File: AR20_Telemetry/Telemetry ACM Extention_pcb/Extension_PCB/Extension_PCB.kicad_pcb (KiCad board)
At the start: 2 copper layers, 55 x 75.5 mm, 9 parts, among them IC1 MCP25625T-E_ML

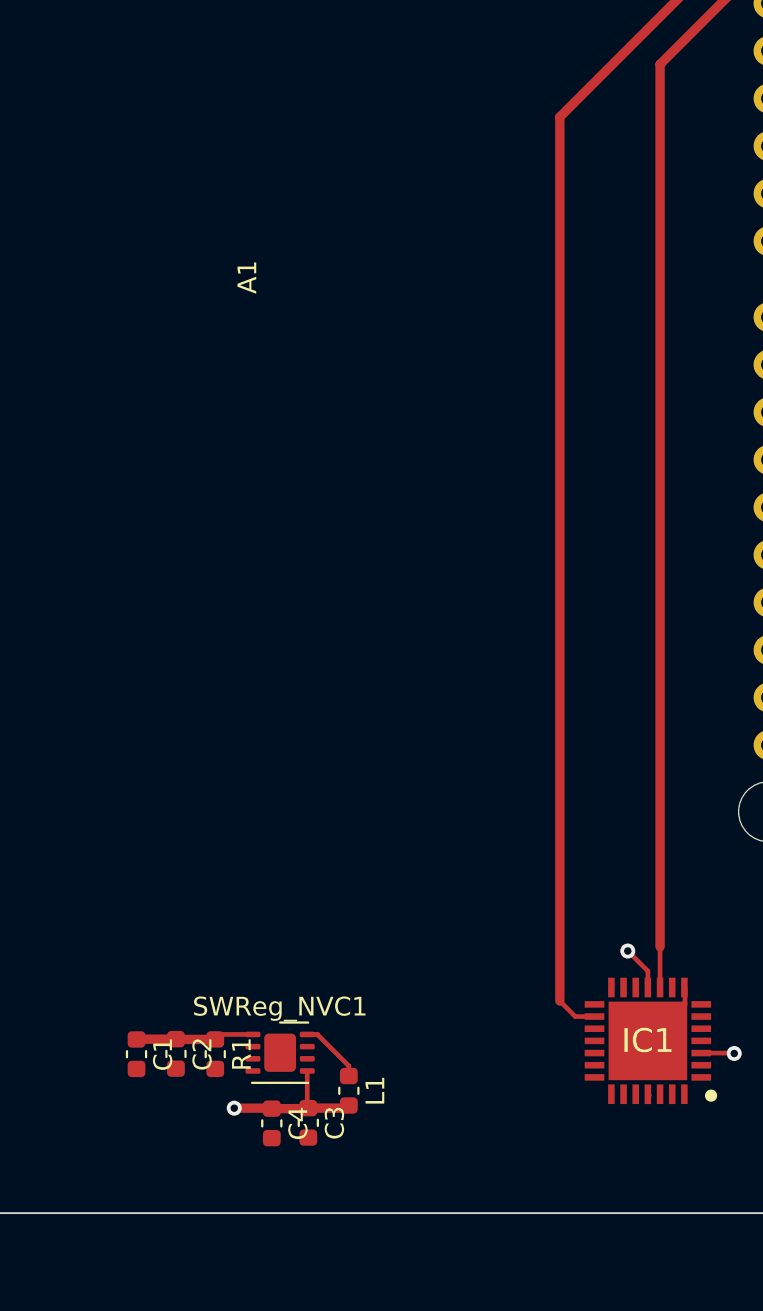
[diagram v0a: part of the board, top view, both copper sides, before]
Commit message: Edited
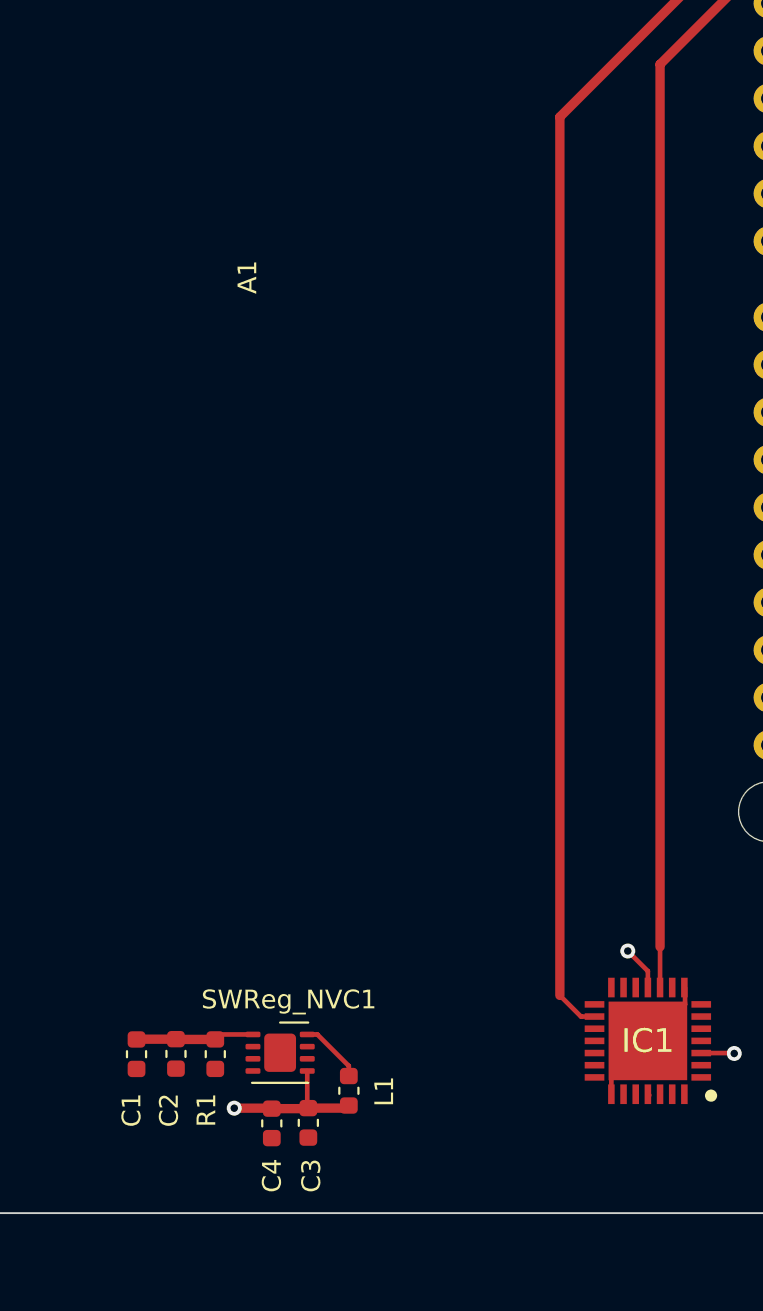
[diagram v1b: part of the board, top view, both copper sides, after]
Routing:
- net Ground: track 3.66 -> 7.32 mm
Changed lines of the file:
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@@
     (thickness 1.6)
     (drawings 4)
-    (tracks 37)
+    (tracks 39)
     (zones 0)
     (modules 9)
@@
     (47 F.CrtYd user)
     (48 B.Fab user)
-    (49 F.Fab user)
+    (49 F.Fab user hide)
   )
   (setup
@@
       (effects (font (size 1.27 1.27) (thickness 0.254)))
     )
-    (fp_text value MCP25625T-E_ML (at 0 0) (layer F.SilkS) hide
+    (fp_text value MCP25625T-E_ML (at 0.57366 -5.19992) (layer F.SilkS) hide
       (effects (font (size 1.27 1.27) (thickness 0.254)))
     )
@@
     (tags "DFN DFN_QFN")
     (attr smd)
-    (fp_text reference SWReg_NVC1 (at 0 -2.45) (layer F.SilkS)
-      (effects (font (size 1 1) (thickness 0.15)))
-    )
-    (fp_text value NCV890430MW50TXG (at 0.6663 7.2878) (layer F.Fab)
-      (effects (font (size 1 1) (thickness 0.15)))
-    )
-    (fp_text user %R (at 0 0) (layer F.Fab)
+    (fp_text reference SWReg_NVC1 (at 0.47152 -2.832) (layer F.SilkS)
+      (effects (font (size 1 1) (thickness 0.15)))
+    )
+    (fp_text value NCV890430MW50TXG (at -0.42848 -6.432) (layer F.Fab)
+      (effects (font (size 1 1) (thickness 0.15)))
+    )
+    (fp_text user %R (at 7.07152 -1.432) (layer F.Fab)
       (effects (font (size 0.75 0.75) (thickness 0.11)))
     )
@@
     (tags resistor)
     (attr smd)
-    (fp_text reference R1 (at 0 -1.43 90) (layer F.SilkS)
-      (effects (font (size 1 1) (thickness 0.15)))
-    )
-    (fp_text value 10k (at 0 1.43 90) (layer F.Fab)
+    (fp_text reference R1 (at 2.99136 0.46474 90) (layer F.SilkS)
+      (effects (font (size 1 1) (thickness 0.15)))
+    )
+    (fp_text value 10k (at -3.00864 -0.03526 90) (layer F.Fab)
       (effects (font (size 1 1) (thickness 0.15)))
     )
@@
     (tags inductor)
     (attr smd)
-    (fp_text reference L1 (at 0 -1.43 90) (layer F.SilkS)
-      (effects (font (size 1 1) (thickness 0.15)))
-    )
-    (fp_text value 2.2u (at 0 1.43 90) (layer F.Fab)
+    (fp_text reference L1 (at 0.03556 -1.9004 90) (layer F.SilkS)
+      (effects (font (size 1 1) (thickness 0.15)))
+    )
+    (fp_text value 2.2u (at 0 -3.4004 90) (layer F.Fab)
       (effects (font (size 1 1) (thickness 0.15)))
     )
@@
     (tags capacitor)
     (attr smd)
-    (fp_text reference C4 (at 0 -1.43 90) (layer F.SilkS)
-      (effects (font (size 1 1) (thickness 0.15)))
-    )
-    (fp_text value 10u (at 0 1.43 90) (layer F.Fab)
-      (effects (font (size 1 1) (thickness 0.15)))
-    )
-    (fp_text user %R (at 0 0 90) (layer F.Fab)
+    (fp_text reference C4 (at 2.79312 -0.0152 90) (layer F.SilkS)
+      (effects (font (size 1 1) (thickness 0.15)))
+    )
+    (fp_text value 10u (at 2.29312 1.9848 90) (layer F.Fab)
+      (effects (font (size 1 1) (thickness 0.15)))
+    )
+    (fp_text user %R (at 0.19312 1.2848 90) (layer F.Fab)
       (effects (font (size 0.4 0.4) (thickness 0.06)))
     )
@@
     (tags capacitor)
     (attr smd)
-    (fp_text reference C3 (at 0 -1.43 90) (layer F.SilkS)
-      (effects (font (size 1 1) (thickness 0.15)))
-    )
-    (fp_text value 0.1u (at 0 1.43 90) (layer F.Fab)
+    (fp_text reference C3 (at 2.82086 -0.16448 90) (layer F.SilkS)
+      (effects (font (size 1 1) (thickness 0.15)))
+    )
+    (fp_text value 0.1u (at 2.82086 -0.06448 90) (layer F.Fab)
       (effects (font (size 0.7 0.7) (thickness 0.1)))
     )
-    (fp_text user %R (at 0 0 90) (layer F.Fab)
+    (fp_text user %R (at 0.02086 -1.16448 90) (layer F.Fab)
       (effects (font (size 0.4 0.4) (thickness 0.06)))
     )
@@
     (tags capacitor)
     (attr smd)
-    (fp_text reference C2 (at 0 -1.43 90) (layer F.SilkS)
-      (effects (font (size 1 1) (thickness 0.15)))
-    )
-    (fp_text value 0.1u (at 0 1.43 90) (layer F.Fab)
+    (fp_text reference C2 (at 3.00386 0.36416 90) (layer F.SilkS)
+      (effects (font (size 1 1) (thickness 0.15)))
+    )
+    (fp_text value 0.1u (at -3.49614 -0.13584 90) (layer F.Fab)
       (effects (font (size 1 1) (thickness 0.15)))
     )
@@
     (tags capacitor)
     (attr smd)
-    (fp_text reference C1 (at 0 -1.43 90) (layer F.SilkS)
-      (effects (font (size 1 1) (thickness 0.15)))
-    )
-    (fp_text value 10u (at 0 1.43 90) (layer F.Fab)
+    (fp_text reference C1 (at 2.98862 0.2585 90) (layer F.SilkS)
+      (effects (font (size 1 1) (thickness 0.15)))
+    )
+    (fp_text value 10u (at -3.01138 0.2585 90) (layer F.Fab)
       (effects (font (size 1 1) (thickness 0.15)))
     )
@@
   (gr_line (start 145 147) (end 200 147) (layer Edge.Cuts) (width 0.1))
   (gr_line (start 145 71.5) (end 145 147) (layer Edge.Cuts) (width 0.1))
+  (segment (start 190.6524 140.70342) (end 190.60922 140.66024) (width 0.25) (layer F.Cu) (net 0))
+  (segment (start 187.73406 137.1854) (end 187.75922 137.16024) (width 0.25) (layer F.Cu) (net 0))
   (segment (start 192.55922 135.86024) (end 190.60922 137.81024) (width 0.25) (layer F.Cu) (net 1))
   (segment (start 192.55922 134.96024) (end 192.55922 135.86024) (width 0.25) (layer F.Cu) (net 1))
+  (segment (start 188.62366 139.75008) (end 190.57366 137.80008) (width 0.25) (layer F.Cu) (net 1))
+  (segment (start 188.62366 140.65008) (end 188.62366 139.75008) (width 0.25) (layer F.Cu) (net 1))
   (segment (start 165.37666 137.72114) (end 165.36416 137.70864) (width 0.5) (layer F.Cu) (net 2))
   (segment (start 167.46474 137.72114) (end 165.37666 137.72114) (width 0.5) (layer F.Cu) (net 2))
   (segment (start 163.27374 137.70864) (end 163.2585 137.72388) (width 0.5) (layer F.Cu) (net 2))
   (segment (start 165.36416 137.70864) (end 163.27374 137.70864) (width 0.5) (layer F.Cu) (net 2))
-  (segment (start 174.5869 139.66424) (end 174.5996 139.67694) (width 0.5) (layer F.Cu) (net 3))
-  (via (at 195.1863 138.47318) (size 0.8) (drill 0.4) (layers F.Cu B.Cu) (net 7))
-  (via (at 168.4782 141.39418) (size 0.8) (drill 0.4) (layers F.Cu B.Cu) (net 7))
-  (segment (start 190.6524 140.70342) (end 190.60922 140.66024) (width 0.25) (layer F.Cu) (net 0))
-  (segment (start 187.73406 137.1854) (end 187.75922 137.16024) (width 0.25) (layer F.Cu) (net 0))
   (segment (start 167.72888 137.457) (end 167.46474 137.72114) (width 0.25) (layer F.Cu) (net 2))
   (segment (start 169.47848 137.457) (end 167.72888 137.457) (width 0.25) (layer F.Cu) (net 2))
+  (segment (start 174.5869 139.66424) (end 174.5996 139.67694) (width 0.5) (layer F.Cu) (net 3))
   (segment (start 174.5996 139.13944) (end 174.5996 139.67694) (width 0.25) (layer F.Cu) (net 3))
   (segment (start 172.91716 137.457) (end 174.5996 139.13944) (width 0.25) (layer F.Cu) (net 3))
@@
   (segment (start 191.22366 132.77634) (end 191.22366 85.63634) (width 0.5) (layer F.Cu) (net 5))
   (segment (start 196.220181 78.099819) (end 197.02018 77.29982) (width 0.5) (layer F.Cu) (net 6))
+  (segment (start 185.87212 135.37212) (end 185.87212 88.44788) (width 0.5) (layer F.Cu) (net 6))
   (segment (start 185.87212 88.44788) (end 196.220181 78.099819) (width 0.5) (layer F.Cu) (net 6))
-  (segment (start 185.87212 135.67354) (end 185.87212 88.44788) (width 0.5) (layer F.Cu) (net 6))
-  (segment (start 186.69866 136.50008) (end 185.87212 135.67354) (width 0.25) (layer F.Cu) (net 6))
-  (segment (start 187.72366 136.50008) (end 186.69866 136.50008) (width 0.25) (layer F.Cu) (net 6))
+  (segment (start 187.00008 136.50008) (end 185.87212 135.37212) (width 0.25) (layer F.Cu) (net 6))
+  (segment (start 187.72366 136.50008) (end 187.00008 136.50008) (width 0.25) (layer F.Cu) (net 6))
+  (via (at 195.1863 138.47318) (size 0.8) (drill 0.4) (layers F.Cu B.Cu) (net 7))
+  (via (at 168.4782 141.39418) (size 0.8) (drill 0.4) (layers F.Cu B.Cu) (net 7))
   (segment (start 170.4596 141.39418) (end 170.4848 141.41938) (width 0.5) (layer F.Cu) (net 7))
   (segment (start 168.4782 141.39418) (end 170.4596 141.39418) (width 0.5) (layer F.Cu) (net 7))

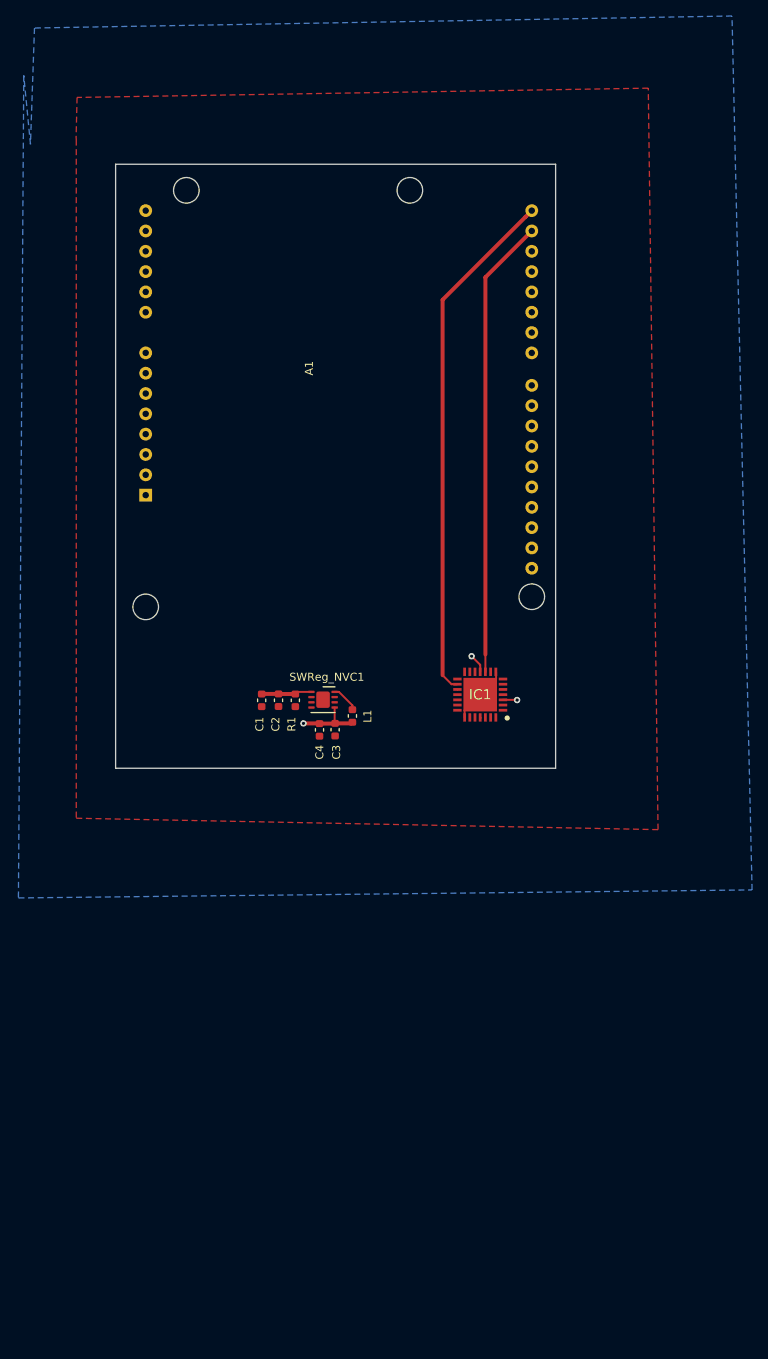
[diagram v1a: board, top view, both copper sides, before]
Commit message: Connector added
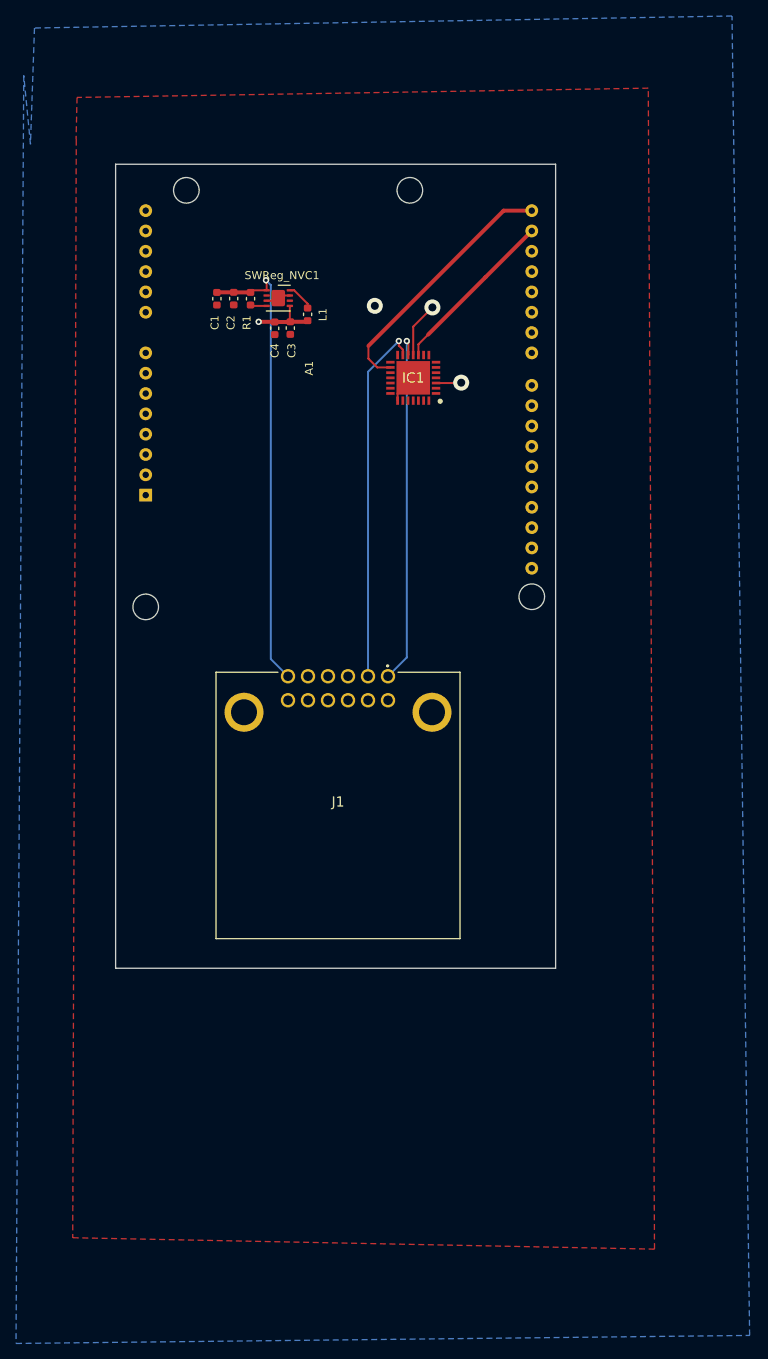
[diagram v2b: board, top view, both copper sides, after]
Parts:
- added J1: MX23A12NF1, MCP25625_Breakoutboard:MX23A12NF1, F.Cu at (172.8, 151.2)
- moved C4 50.5 mm to (164.9, 92.0)
- moved R1 50.5 mm to (161.9, 88.3)
- moved C1 50.5 mm to (157.7, 88.3)
- moved C2 50.5 mm to (159.8, 88.3)
- moved L1 50.5 mm to (169.0, 90.3)
- moved C3 50.5 mm to (166.8, 92.0)
- moved SWReg_NVC1 50.5 mm to (165.3, 88.2)
- moved IC1 40.5 mm to (182.2, 98.2)
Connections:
- IC1 pad 12: (no net) -> CANL
- IC1 pad 13: (no net) -> CANH
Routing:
- net 12V_IN: track 6.34 -> 58.3 mm, vias 0 -> 1
- net CANH: track 0.00 -> 45.5 mm, vias 0 -> 1
- net CANL: track 0.00 -> 44.7 mm, vias 0 -> 1
- net TX_4G: track 57.5 -> 22.0 mm
- net RX_4G: track 65.0 -> 32.2 mm
- net Vinn_5V: track 12.4 -> 18.3 mm, vias 3 -> 4
- net Net-(R1-Pad2): track 0.00 -> 2.06 mm
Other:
- board size 55 x 75.5 mm -> 55 x 100.5 mm
